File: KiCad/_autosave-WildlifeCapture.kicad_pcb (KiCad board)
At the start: 2 copper layers, 105 x 135 mm, 32 parts, among them P1 ANALOG, P1 USB_A, P2 GPS, P2 USB_B, P7 PROGRAM, P8 DIGITAL IO, SW1 A, SW1 RESET, SW2 BUTTON, SW2 LEADSW, U1 IM920_interplan, U1 Mini360, U3 ESP-WROOM-32, U3 STM32F103C8T6MinimumDevelopBo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, U4 RASPBERRYPI_GPIO_40

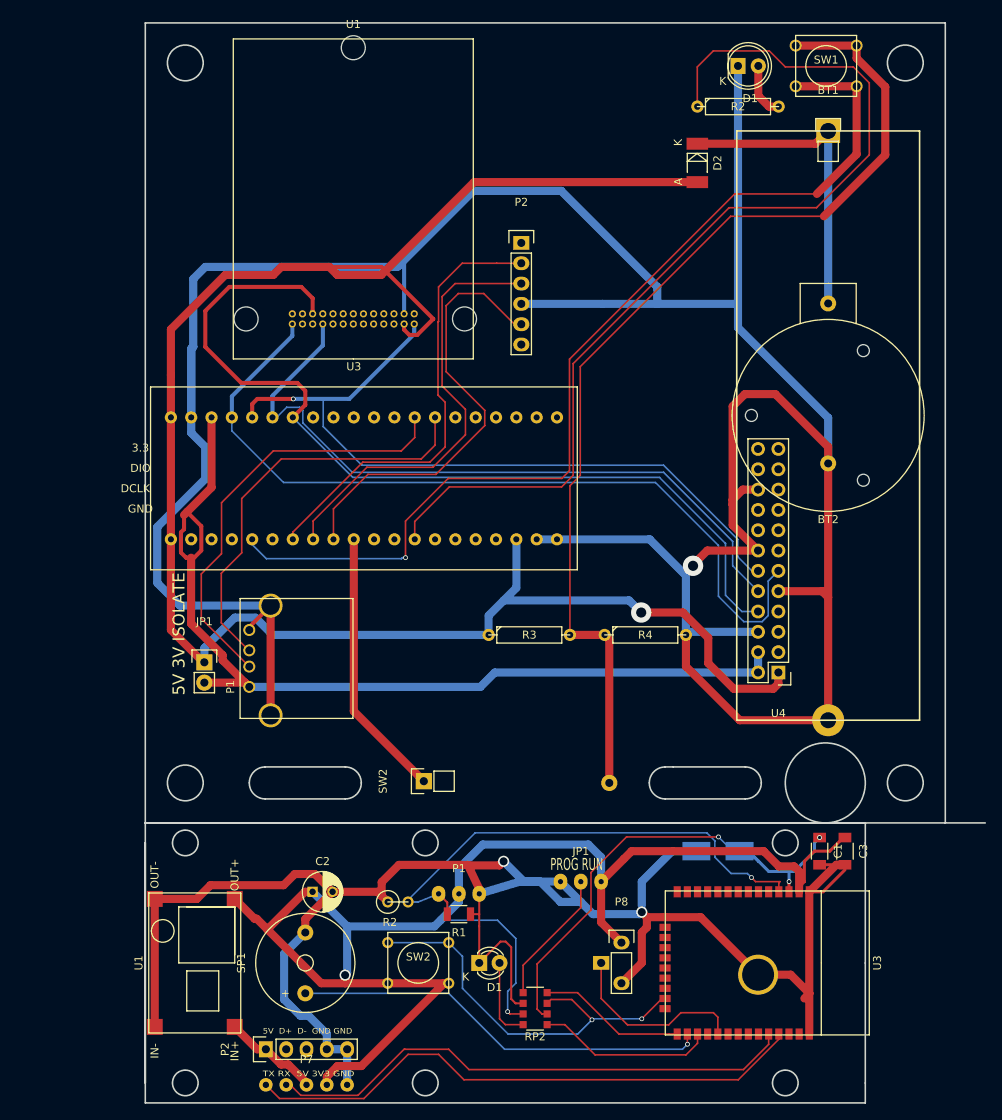
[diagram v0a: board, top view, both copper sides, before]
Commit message: Change to Take 2
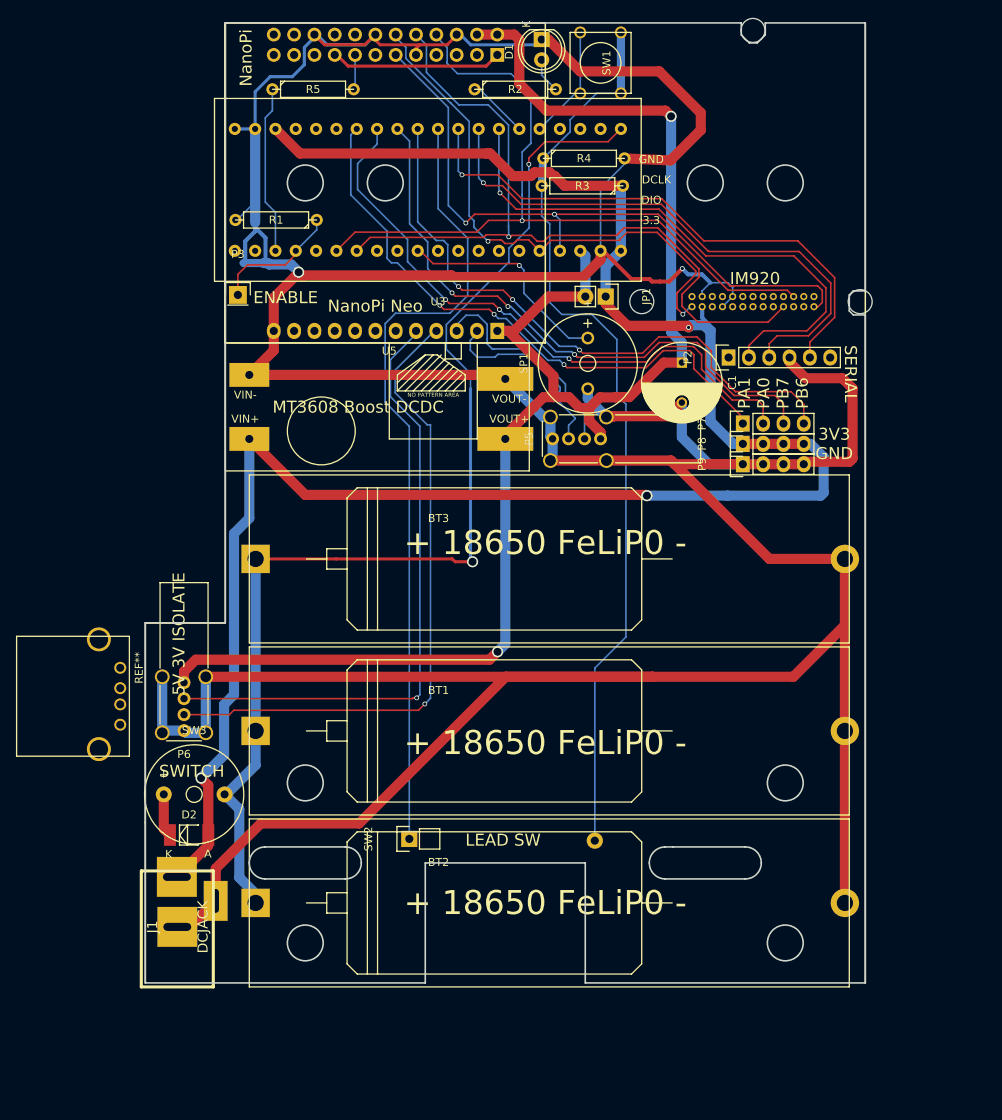
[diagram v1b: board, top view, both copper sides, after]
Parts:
- removed C2: CP1, Capacitors_ThroughHole:C_Radial_D5_L11_P2.5
- removed C3: 0.1uF, library:C_1206_HandSoldering_Small
- removed the D1 at (132.8, 153.7)
- removed the JP1 at (145.5, 143.6)
- removed P1: USB_A, Connect:USB_A
- removed P1: ANALOG, library:SolderWirePad_Oval_3xInline_0-65mmDrill
- removed the P2 at (106.2, 164.5)
- removed the R2 at (122.7, 146.1)
- removed RP2: R_PACK4, Resistors_SMD:R_Array_Convex_4x1206
- removed the SW1 at (162.7, 139.8)
- removed the SW2 at (125.2, 153.7)
- removed the U1 at (97.3, 153.7)
- removed the U3 at (174.1, 153.7)
- added BT3: Battery, library:18650BatteryCase, F.Cu at (134.1, 103.2)
- added J1: DCJACK, library:DCJACK, F.Cu at (95.1, 149.2)
- added P3: EN, Pin_Headers:Pin_Header_Straight_1x01, F.Cu at (102.7, 70.2)
- added P4: NanoPi_USB/Audio/IR, Pin_Headers:Pin_Header_Straight_1x12, B.Cu at (135.1, 74.7)
- added P5: USB_A, Connect:USB_A_Vertical, F.Cu at (148.0, 88.2)
- added P6: USB_A, Connect:USB_A_Vertical, F.Cu at (95.9, 118.7)
- added P9: GND, Pin_Headers:Pin_Header_Straight_1x04, F.Cu at (165.8, 91.4)
- added R5: R, Discret:R4, F.Cu at (112.1, 44.5)
- added REF**: USB_A, Connect:USB_A, F.Cu at (88.0, 116.9)
- added SW3: SWITCH_INV, Buzzers_Beepers:Buzzer_12x9.5RM7.6, F.Cu at (97.2, 132.7)
- added U5: MT3608, library:MT3608, F.Cu at (120.1, 84.2)
- BT1: footprint Pin_Headers:Pin_Header_Straight_1x02 -> library:18650BatteryCase
- BT2: footprint library:BATTERY_CR2032_CH25-2032LF_CONFORTABLE -> library:18650BatteryCase
- C1: value 0.1uF -> CP1; footprint library:C_1206_HandSoldering_Small -> Capacitors_ThroughHole:C_Radial_D10_L13_P5
- P7: value PROGRAM -> SERVICE; footprint library:SolderWirePad_Circle_5xInline_0-8mmDrill -> Pin_Headers:Pin_Header_Straight_1x04
- P8: value DIGITAL IO -> VCC; footprint Pin_Headers:Pin_Header_Straight_1x03 -> Pin_Headers:Pin_Header_Straight_1x04
- R1: value 4.7kΩ -> R; footprint Resistors_SMD:R_1206 -> Discret:R4
- SP1: footprint Buzzers_Beepers:Buzzer_12x9.5RM7.6 -> Buzzers_Beepers:MagneticBuzzer_ProSignal_ABT-410-RC
- U1, U4: moved to B.Cu
- moved D2 105.3 mm to (96.6, 137.8), turned to 0 degrees
- moved P7 99.0 mm to (165.8, 86.3), turned to 90 degrees
- moved R1 89.7 mm to (107.4, 60.9)
- moved BT1 86.1 mm to (134.1, 124.7)
- moved U4 84.8 mm to (135.1, 40.2), turned to 90 degrees
- moved SP1 80.0 mm to (146.4, 82.0)
- moved BT2 74.2 mm to (134.1, 146.2), turned to 0 degrees
- moved JP1 67.9 mm to (148.6, 70.4), turned to 270 degrees
- moved P8 64.2 mm to (165.8, 88.9), turned to 90 degrees
- moved C1 63.4 mm to (158.2, 78.7)
- moved R4 60.1 mm to (145.9, 53.2)
- moved R3 56.5 mm to (145.7, 56.6), turned to 180 degrees
- moved U1 50.0 mm to (167.0, 71.1), turned to 180 degrees
- moved U3 47.2 mm to (99.7, 68.5), turned to 0 degrees
- moved P2 29.6 mm to (164.0, 78.1), turned to 90 degrees
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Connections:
- C1 pad 1: Net-(C1-Pad1) -> +5V
- D2 pad 1: Net-(BT1-Pad1) -> Net-(D2-Pad1)
- D2 pad 2: +3V3 -> +BATT
- JP1 pad 1: +3V3 -> +BATT
- JP1 pad 2: Net-(JP1-Pad2) -> +5V
- P7 pad 1: Net-(P12-Pad1) -> Net-(P7-Pad1)
- P7 pad 2: Net-(P12-Pad2) -> Net-(P7-Pad2)
- P7 pad 3: +5V -> Net-(P7-Pad3)
- P7 pad 4: +3V3 -> Net-(P7-Pad4)
- P8 pad 1: Net-(P8-Pad1) -> +BATT
- P8 pad 2: +3V3 -> +BATT
- P8 pad 3: GND -> +BATT
- R1 pad 1: GND -> Net-(P3-Pad1)
- R1 pad 2: Net-(P1-Pad1) -> GND
- R3 pad 1: +3V3 -> +BATT
- SP1 pad 1: Net-(SP1-Pad1) -> GND
- SP1 pad 2: GND -> Net-(SP1-Pad2)
- U1 pad 18: Net-(U1-Pad18) -> GND
- U1 pad 19: Net-(U1-Pad19) -> GND
- U1 pad 23: +3V3 -> +BATT
- U3 pad 14: Net-(U1-Pad6) -> Net-(U3-Pad14)
- U3 pad 15: Net-(U1-Pad7) -> Net-(U3-Pad15)
- U3 pad 18: Net-(JP1-Pad2) -> +5V
- U3 pad 20: +3V3 -> +BATT
- U3 pad 21: +3V3 -> Net-(BT1-Pad1)
- U3 pad 26: Net-(U3-Pad26) -> Net-(R2-Pad1)
- U3 pad 31: Net-(U3-Pad31) -> Net-(P7-Pad4)
- U3 pad 32: Net-(U3-Pad32) -> Net-(P7-Pad3)
- U3 pad 33: Net-(R2-Pad1) -> Net-(P7-Pad2)
- U3 pad 34: Net-(U3-Pad34) -> Net-(P7-Pad1)
- U3 pad 38: +3V3 -> +BATT
- U3 pad 4: Net-(U3-Pad4) -> Net-(P3-Pad1)
- U3 pad 6: Net-(U3-Pad6) -> Net-(U1-Pad6)
- U3 pad 7: Net-(P1-Pad3) -> Net-(U1-Pad7)
- U4 pad 17: Net-(U4-Pad17) -> +3V3
- U4 pad 2: Net-(JP1-Pad2) -> +5V
- U4 pad 4: Net-(JP1-Pad2) -> +5V
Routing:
- net +3V3: track 436.1 -> 21.5 mm, vias 3 -> 0
- net +BATT: track 0.00 -> 263.7 mm, vias 0 -> 3
- net +5V: track 12.1 -> 194.3 mm, vias 0 -> 2
- net Net-(JP1-Pad2): track 136.0 -> 0.00 mm
- net Net-(R2-Pad1): track 124.2 -> 7.64 mm
- net Net-(SW1-Pad2): track 124.8 -> 14.5 mm, vias 1 -> 0
- net Net-(BT1-Pad1): track 38.6 -> 142.7 mm, vias 0 -> 2
- net Net-(P4-Pad4): track 0.00 -> 81.9 mm, vias 0 -> 1
- net Net-(P4-Pad5): track 0.00 -> 78.7 mm, vias 0 -> 1
- net Net-(P7-Pad2): track 0.00 -> 77.0 mm, vias 0 -> 3
- net Net-(P7-Pad4): track 0.00 -> 76.9 mm, vias 0 -> 3
- net Net-(P7-Pad3): track 0.00 -> 75.7 mm, vias 0 -> 3
- net Net-(P7-Pad1): track 0.00 -> 74.6 mm, vias 0 -> 3
- net Net-(P12-Pad1): track 71.2 -> 0.00 mm
- net Net-(P12-Pad2): track 66.9 -> 0.00 mm
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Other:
- board size 105 x 135 mm -> 90 x 120 mm
- board text added: "+ 18650 FeLiP0 -"
- board text added: "3V3 GND"
- board text added: "ENABLE"
- board text added: "IM920"
- board text added: "LEAD SW"
- board text added: "MT3608 Boost DCDC"
- board text added: "NanoPi"
- board text added: "NanoPi Neo"
- board text added: "PA1 PA0 PB7 PB6"
- board text added: "SERIAL"
- board text added: "SWITCH"
- board text removed: "5V D+ D- GND GND"
- board text removed: "PROG RUN"
- board text removed: "RUN PROG"
- board text removed: "TX RX 5V 3V3 GND"
